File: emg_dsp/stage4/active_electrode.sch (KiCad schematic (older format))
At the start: 24 parts

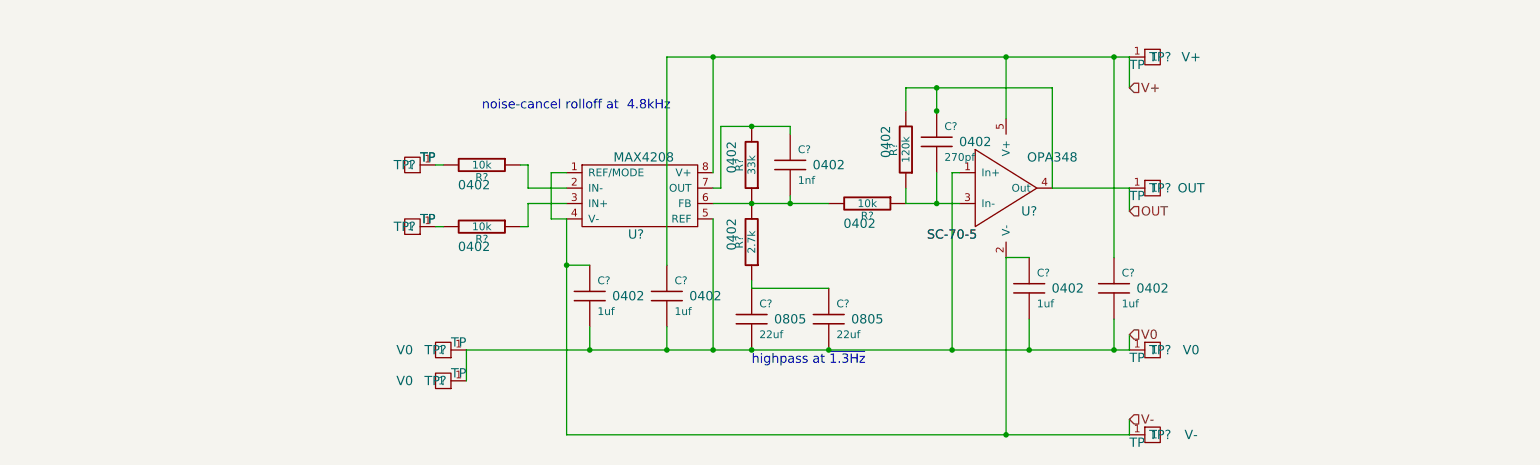
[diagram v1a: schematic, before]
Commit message: notes, schematic mods, etc.
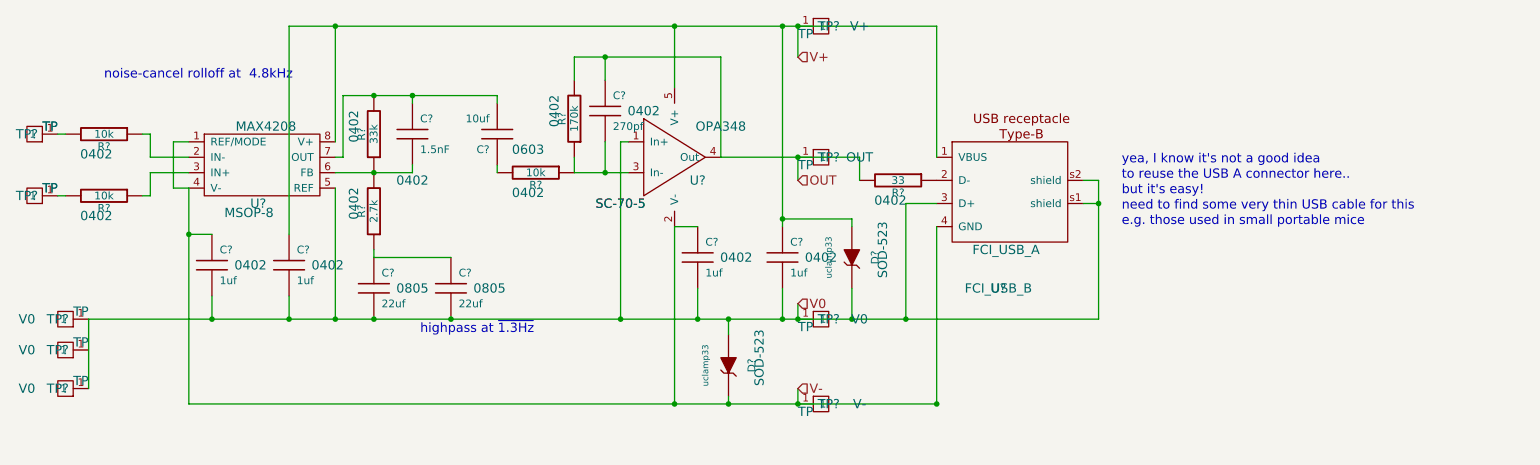
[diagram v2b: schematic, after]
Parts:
- added C?: 10uf, 0603, symbol C
- added D? (x2): uclamp33, SOD-523, symbol ZENER
- added R?: 33, 0402, symbol R
- added TP?: V0, TP, symbol TP
- added U?: FCI_USB_B, FCI_USB_A, symbol FCI_USB_B
- C?: value 1nf -> 1.5nF
- R?: value 120k -> 170k
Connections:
- net OUT: now also R?.2
- net V+: now also D?.1 (A), U?.1 (VBUS)
- net V-: now also D?.2 (K), U?.4 (GND)
- net V0: now also D?.1 (A), D?.2 (K), TP?.1, U?.3 (D+), U?.s1 (shield), U?.s2 (shield); no longer TP?.1
- net at C?.2, R?.1, R?.2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: no longer R?.2
- net at C?.1, R?.2, U?.7 (OUT): now also C?.2
- new net: C?.1, R?.2
- new net: R?.1, U?.2 (D-)
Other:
- note added: "but it's easy!"
- note added: "e.g. those used in small portable mice"
- note added: "need to find some very thin USB cable for this"
- note added: "to reuse the USB A connector here.."
- note added: "yea, I know it's not a good idea"
- moved on the sheet: C?, R?, TP?, U?
